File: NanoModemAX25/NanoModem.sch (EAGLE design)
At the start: 49 parts, among them IC1 FT232RL, Q1 T2N7002AK, X1 MINI-USB-32005-201, Y1 16MHz

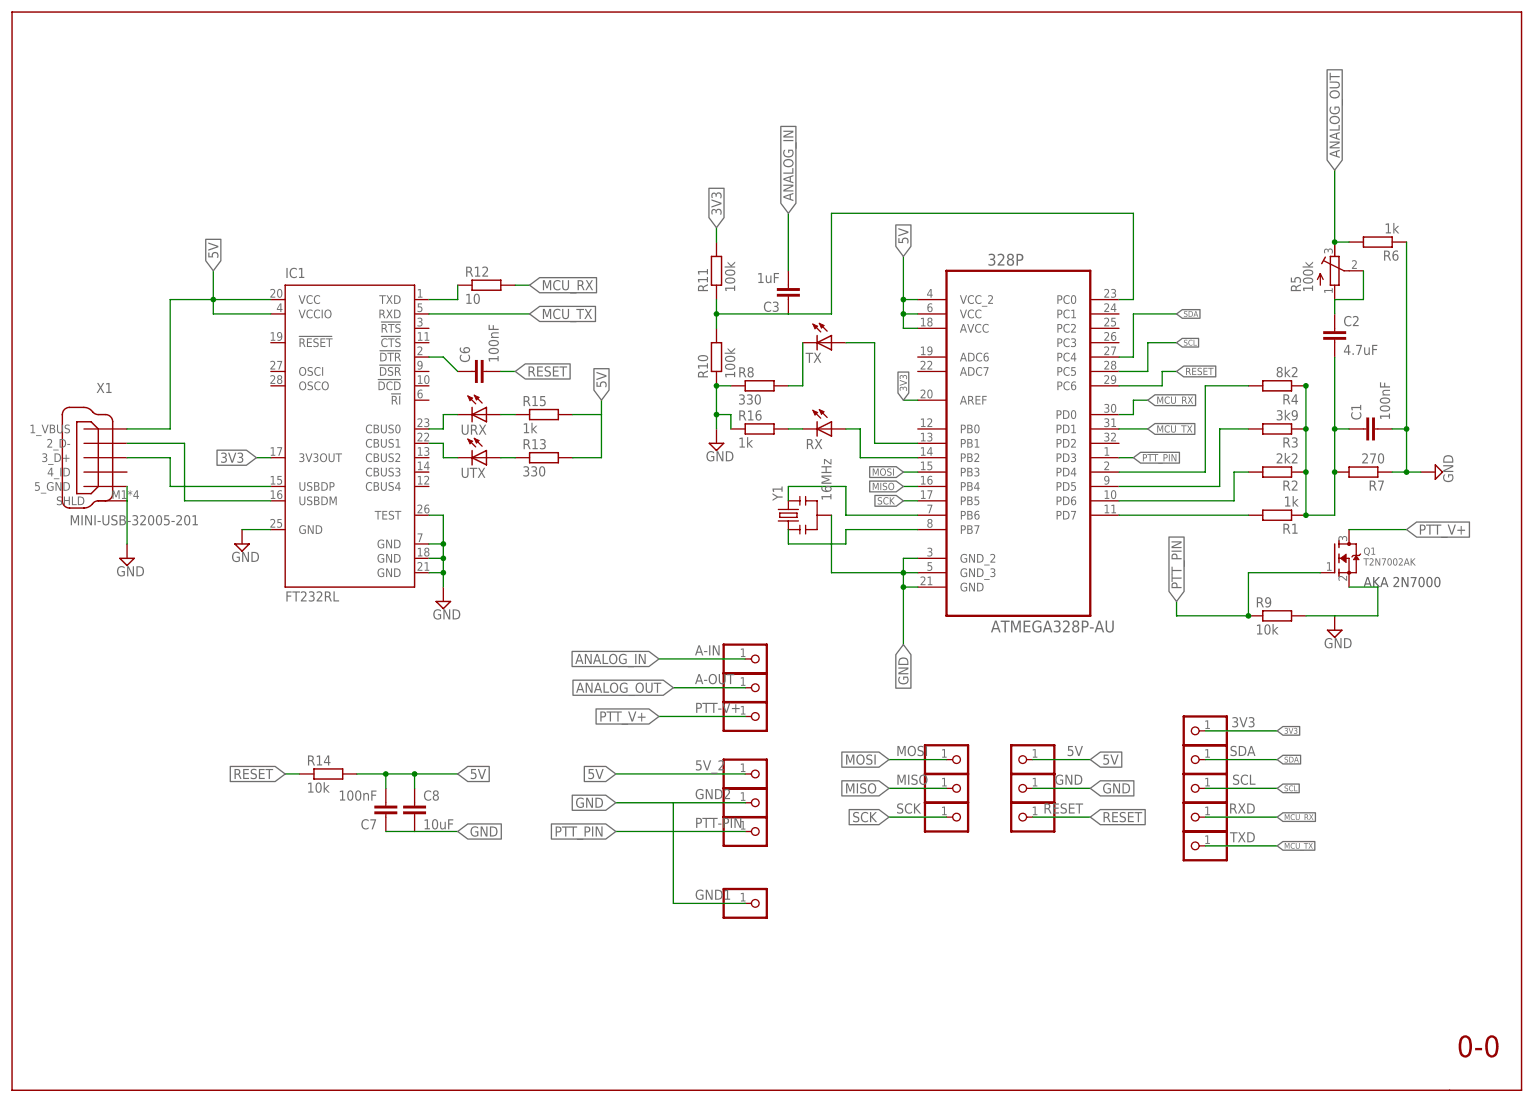
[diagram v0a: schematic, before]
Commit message: some changes to the APRS modem board
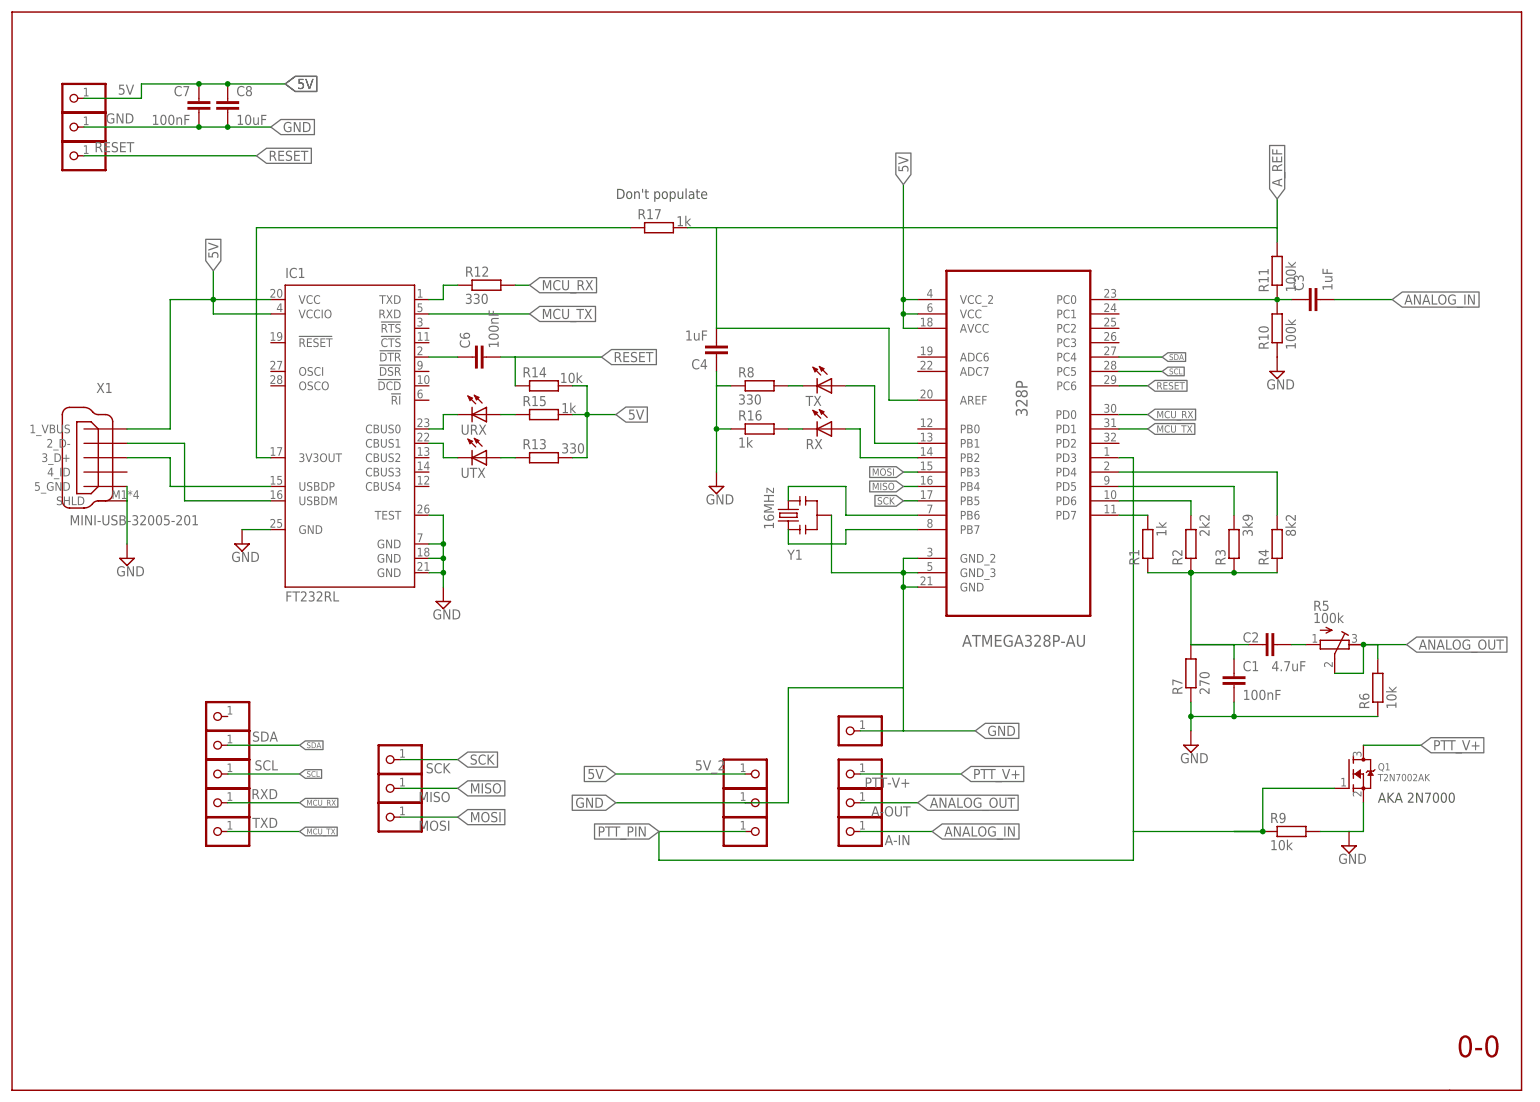
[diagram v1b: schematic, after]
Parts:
- added C4: 1uF, rcl:C-EUC0603
- added R17: 1k, rcl:R-EU_R0603
- C8: device rcl:C-EUC0805 -> rcl:C-EUC1210
- R12: value 10 -> 330
- R6: value 1k -> 10k
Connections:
- removed net N$9: C2.1, R5.A, R5.S
- new net A_REF: 328P.AREF, C4.2, R11.2, R17.2
- new net N$11: C2.1, R5.A
- net 3V3: now also R17.1; no longer 328P.AREF, 3V3.1, R11.2
- net ANALOG_OUT: now also R5.S
- net GND: now also C4.1
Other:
- note added: "Don't populate"
- moved on the sheet: 5V, A-IN, A-OUT, C1, C2, C3, C6, C7, C8, GND, MISO, MOSI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
